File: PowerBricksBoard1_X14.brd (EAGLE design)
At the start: 76.2 x 53.3 mm, 16 parts

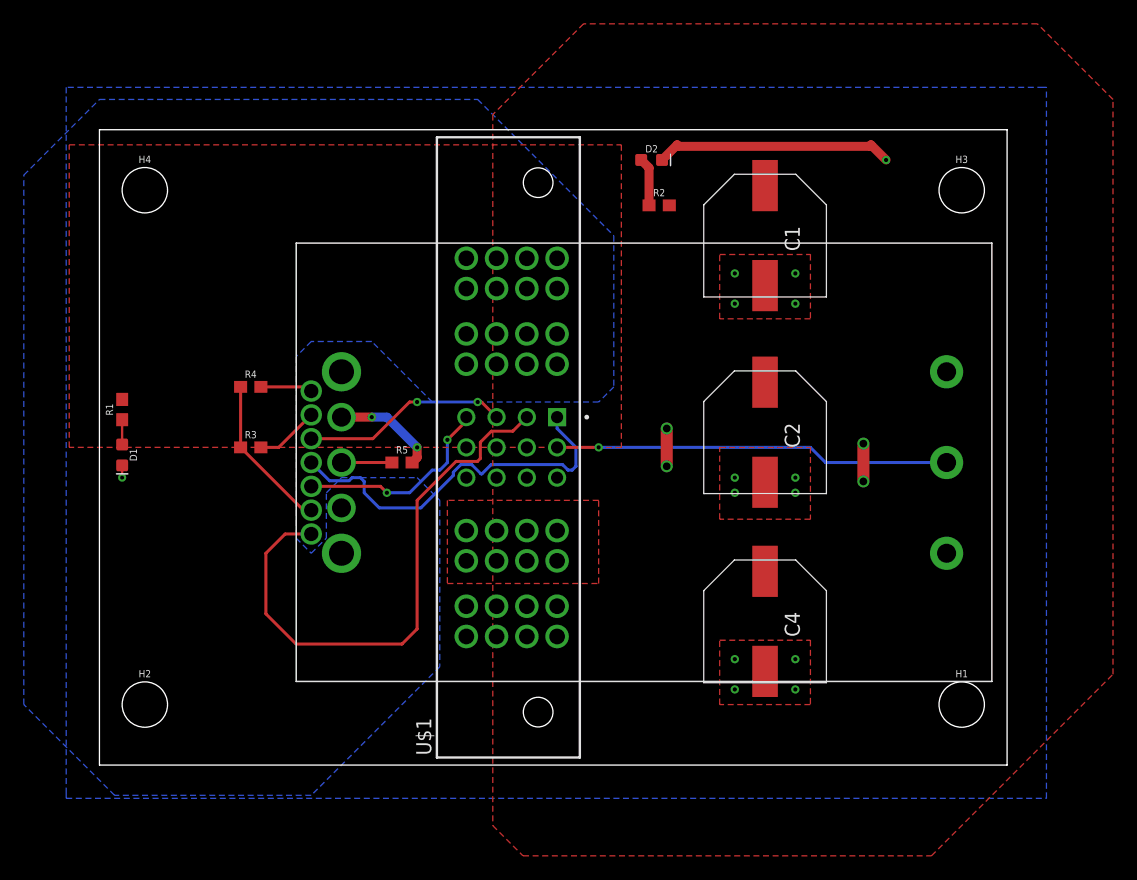
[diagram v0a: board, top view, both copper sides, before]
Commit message: more adjustments
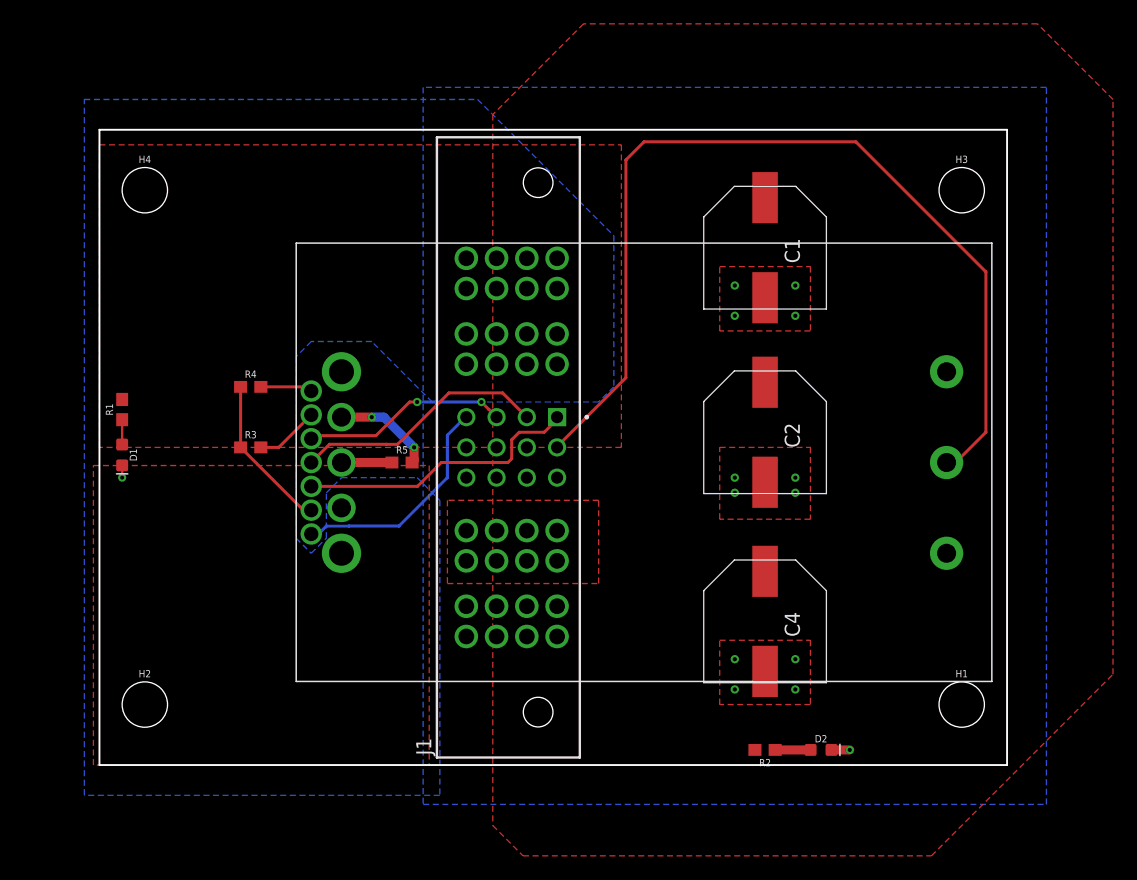
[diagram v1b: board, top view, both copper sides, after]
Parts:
- removed U$1: CONN_BRICKS, CONN, Distribution-Bricks:SAMTEC_PESC-02-12-02-01-X-VT-LC
- added J1: PESC-02-12-02-01-X-VT-LC(BRICKS-DISTRIBUTION), CONN, Distribution-Bricks:SAMTEC_PESC-02-12-02-01-X-VT-LC(B-D)
- moved D2 51.5 mm to (60.6, 0.00)
- moved R2 46.6 mm to (55.9, 0.00), turned to 180 degrees
- moved C1 1.02 mm to (55.9, 42.2)
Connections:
- net 12V: now also J1.P01_1, J1.P01_2, J1.P01_3, J1.P01_4, J1.P01_5, J1.P01_6, J1.P01_7, J1.P01_8; no longer U$1.P01_1, U$1.P01_2, U$1.P01_3, U$1.P01_4, U$1.P01_5, U$1.P01_6, U$1.P01_7, U$1.P01_8
- net 12_GND: now also J1.P02_1, J1.P02_2, J1.P02_3, J1.P02_4, J1.P02_5, J1.P02_6, J1.P02_7, J1.P02_8; no longer U$1.P02_1, U$1.P02_2, U$1.P02_3, U$1.P02_4, U$1.P02_5, U$1.P02_6, U$1.P02_7, U$1.P02_8
- net 48V: now also J1.P03_1, J1.P03_2, J1.P03_3, J1.P03_4, J1.P03_5, J1.P03_6, J1.P03_7, J1.P03_8; no longer U$1.P03_1, U$1.P03_2, U$1.P03_3, U$1.P03_4, U$1.P03_5, U$1.P03_6, U$1.P03_7, U$1.P03_8
- net 48_GND: now also J1.P04_1, J1.P04_2, J1.P04_3, J1.P04_4, J1.P04_5, J1.P04_6, J1.P04_7, J1.P04_8; no longer U$1.P04_1, U$1.P04_2, U$1.P04_3, U$1.P04_4, U$1.P04_5, U$1.P04_6, U$1.P04_7, U$1.P04_8
- net ALERT: now also J1.02; no longer U$1.01
- net C2: now also J1.04; no longer U$1.02
- net CLK: now also J1.03; no longer U$1.03
- net DATA: now also J1.01; no longer U$1.04
- net ON/OFF: now also J1.05; no longer U$1.05
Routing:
- net ON/OFF: track 33.2 -> 79.7 mm, vias 1 -> 0
- net C2: track 47.5 -> 19.2 mm
- net 48_GND: track 26.5 -> 1.54 mm, vias 17 -> 13
- net ALERT: track 32.0 -> 21.4 mm
- net DATA: track 17.2 -> 24.1 mm, vias 2 -> 0
- net N$2: track 4.08 -> 2.97 mm
- added copper zone on layer 1, net 12_GND
